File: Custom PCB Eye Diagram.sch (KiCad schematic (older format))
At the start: 61 parts, among them IC1 DSC1123CI2-125.0000, J1 Conn_01x02, J10 PJ-102B, J11 Conn_01x02, J12 Conn_01x02, J13 47272-0001, J14 LSHM-150-XX.X-XX-DV-A-N, J15 Conn_01x02, J16 LSHM-150-XX.X-XX-DV-A-N, J17 Conn_01x02, J2 Conn_01x04, J3 Conn_01x03, J4 Conn_01x02, J5 Conn_01x04, J6 0878321420, J7 Conn_01x02, J8 Conn_01x02, J9 47272-0001, U1 OKI-78SR-3.3_1.5-W36-C

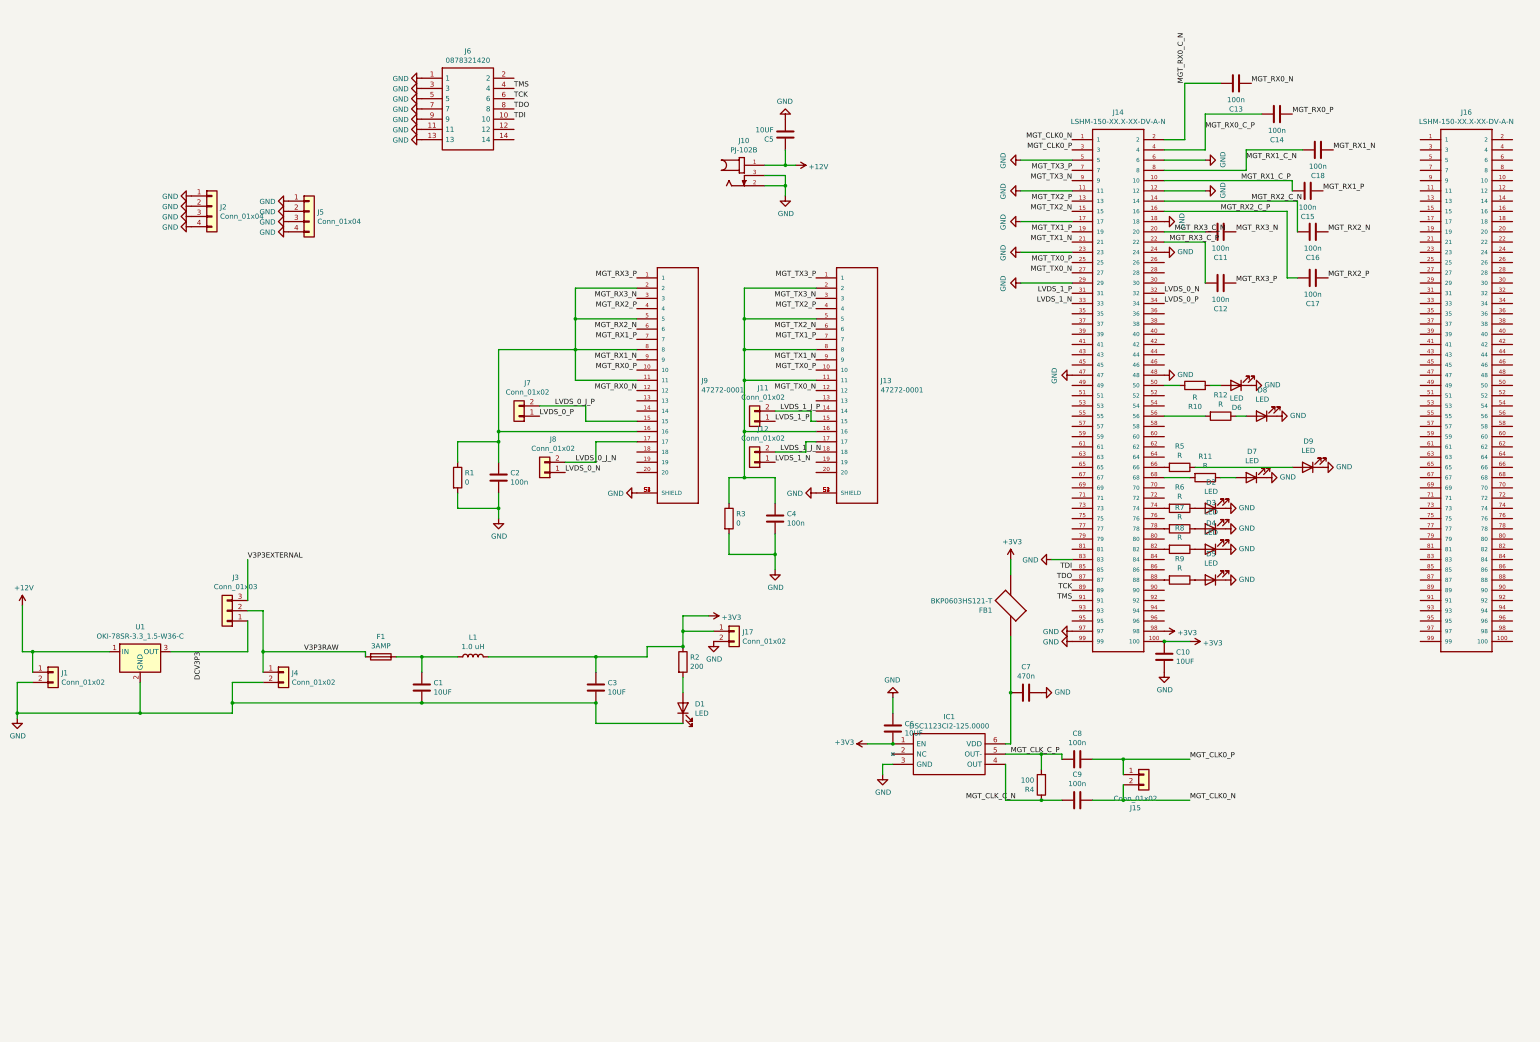
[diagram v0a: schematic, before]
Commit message: PCB 2.0
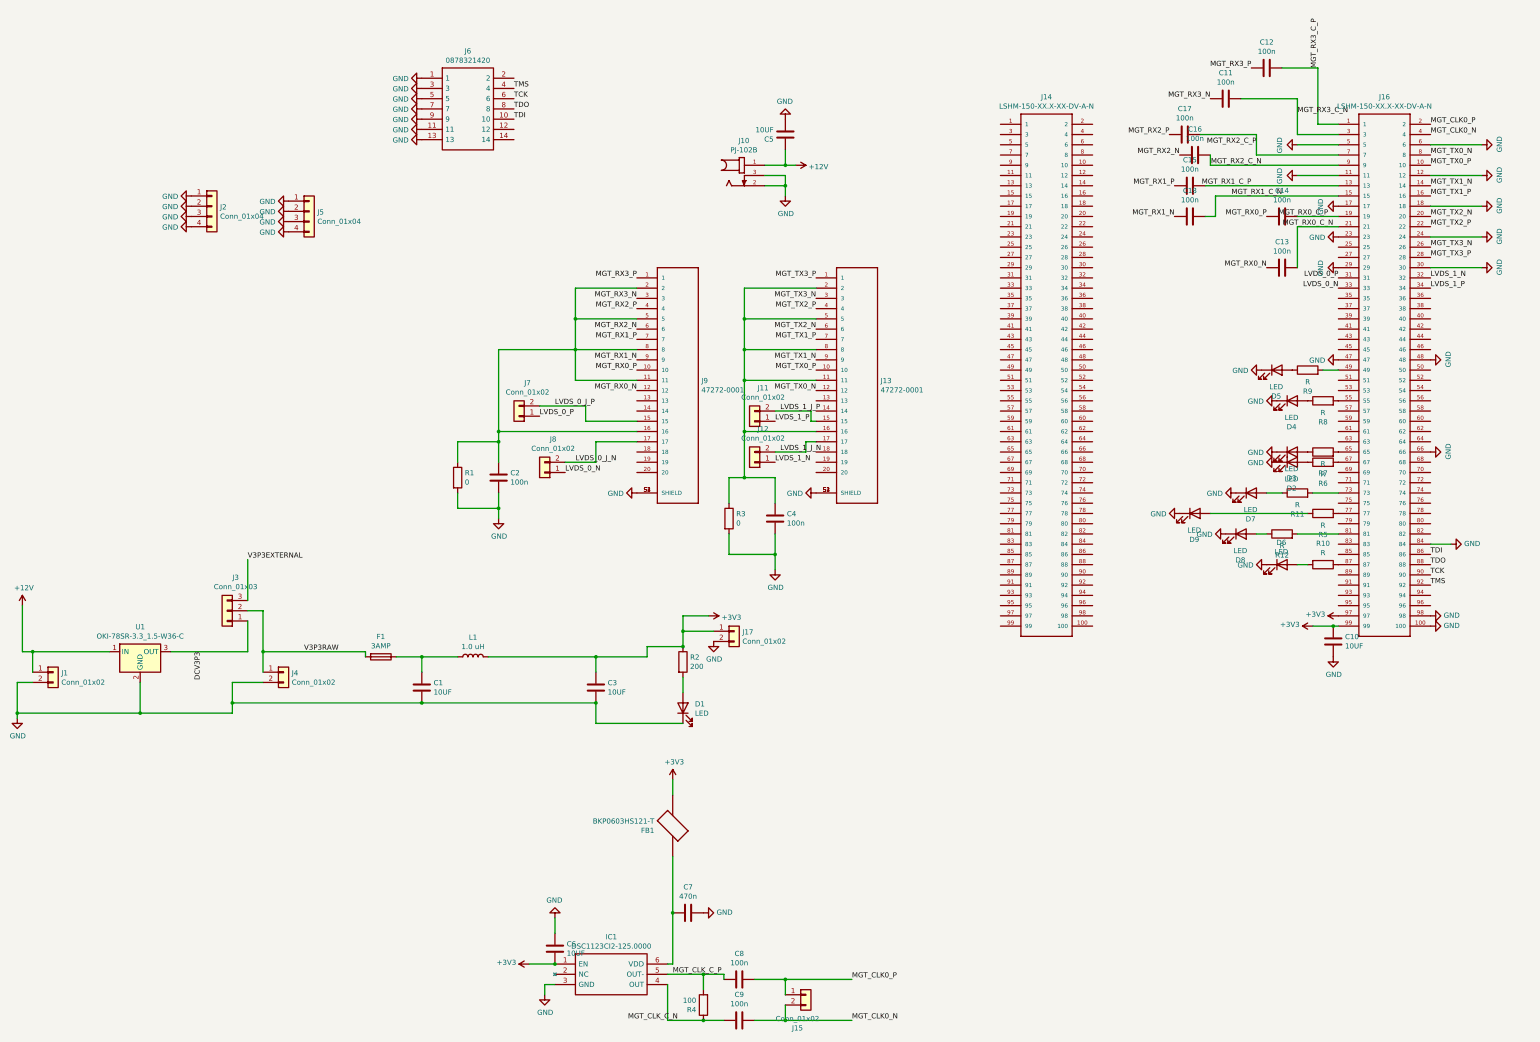
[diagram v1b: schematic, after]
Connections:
- net +3V3: now also J16.97, J16.99; no longer J14.100, J14.98
- net GND: now also J16.100, J16.11, J16.12, J16.17, J16.18, J16.23, J16.24, J16.29, J16.30, J16.47, J16.48, J16.5, J16.6, J16.66, J16.84, J16.98; no longer J14.11, J14.12, J14.17, J14.18, J14.23, J14.24, J14.29, J14.47, J14.48, J14.5, J14.6, J14.83, J14.97, J14.99
- net LVDS_0_N: now also J16.33; no longer J14.32
- net LVDS_0_P: now also J16.31; no longer J14.34
- net LVDS_1_N: now also J16.32; no longer J14.33
- net LVDS_1_P: now also J16.34; no longer J14.31
- net MGT_CLK0_N: now also J16.4; no longer J14.1
- net MGT_CLK0_P: now also J16.2; no longer J14.3
- net MGT_RX0_C_N: now also J16.21; no longer J14.2
- net MGT_RX0_C_P: now also J16.19; no longer J14.4
- net MGT_RX1_C_N: now also J16.15; no longer J14.8
- net MGT_RX1_C_P: now also J16.13; no longer J14.10
- net MGT_RX2_C_N: now also J16.9; no longer J14.14
- net MGT_RX2_C_P: now also J16.7; no longer J14.16
- net MGT_RX3_C_N: now also J16.3; no longer J14.20
- net MGT_RX3_C_P: now also J16.1; no longer J14.22
- net MGT_TX0_N: now also J16.8; no longer J14.27
- net MGT_TX0_P: now also J16.10; no longer J14.25
- net MGT_TX1_N: now also J16.14; no longer J14.21
- net MGT_TX1_P: now also J16.16; no longer J14.19
- net MGT_TX2_N: now also J16.20; no longer J14.15
- net MGT_TX2_P: now also J16.22; no longer J14.13
- net MGT_TX3_N: now also J16.26; no longer J14.9
- net MGT_TX3_P: now also J16.28; no longer J14.7
- net TCK: now also J16.90; no longer J14.89
- net TDI: now also J16.86; no longer J14.85
- net TDO: now also J16.88; no longer J14.87
- net TMS: now also J16.92; no longer J14.91
- net at J14.50: no longer R10.1
- net at J14.56: no longer R12.2
- net at J14.66: no longer R5.2
- net at J14.68: no longer R11.2
- net at J14.74: no longer R6.2
- net at J14.78: no longer R7.2
- net at J14.82: no longer R8.2
- net at J14.88: no longer R9.2
- net at J16.49: now also R9.2
- net at J16.55: now also R8.2
- net at J16.65: now also R7.2
- net at J16.67: now also R6.2
- net at J16.73: now also R11.2
- net at J16.77: now also R5.2
- net at J16.81: now also R12.2
- net at J16.87: now also R10.1
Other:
- moved on the sheet: C10, C11, C12, C13, C14, C15, C16, C17, C18, C6, C7, C8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
